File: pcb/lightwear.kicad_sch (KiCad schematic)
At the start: 21 parts, among them SW1 SW_SPST

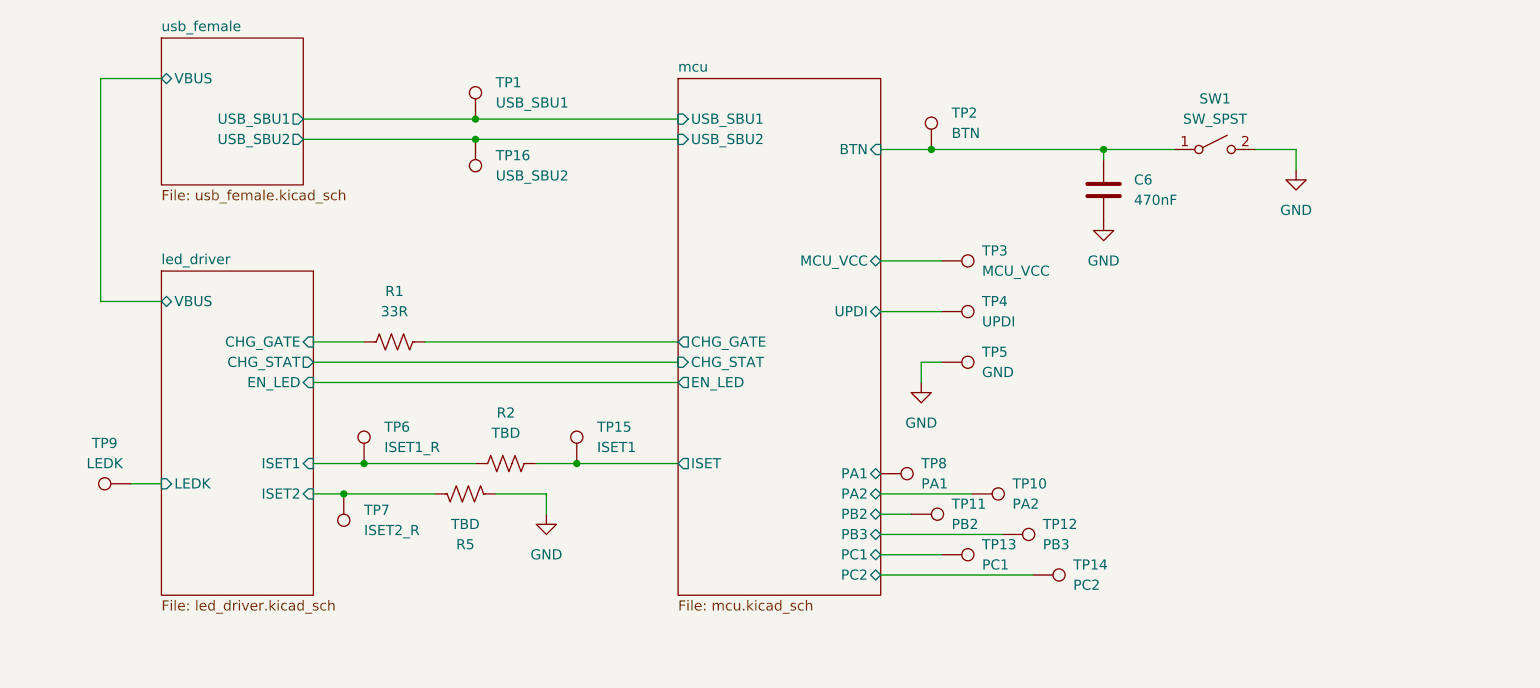
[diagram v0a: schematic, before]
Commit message: rev0 done
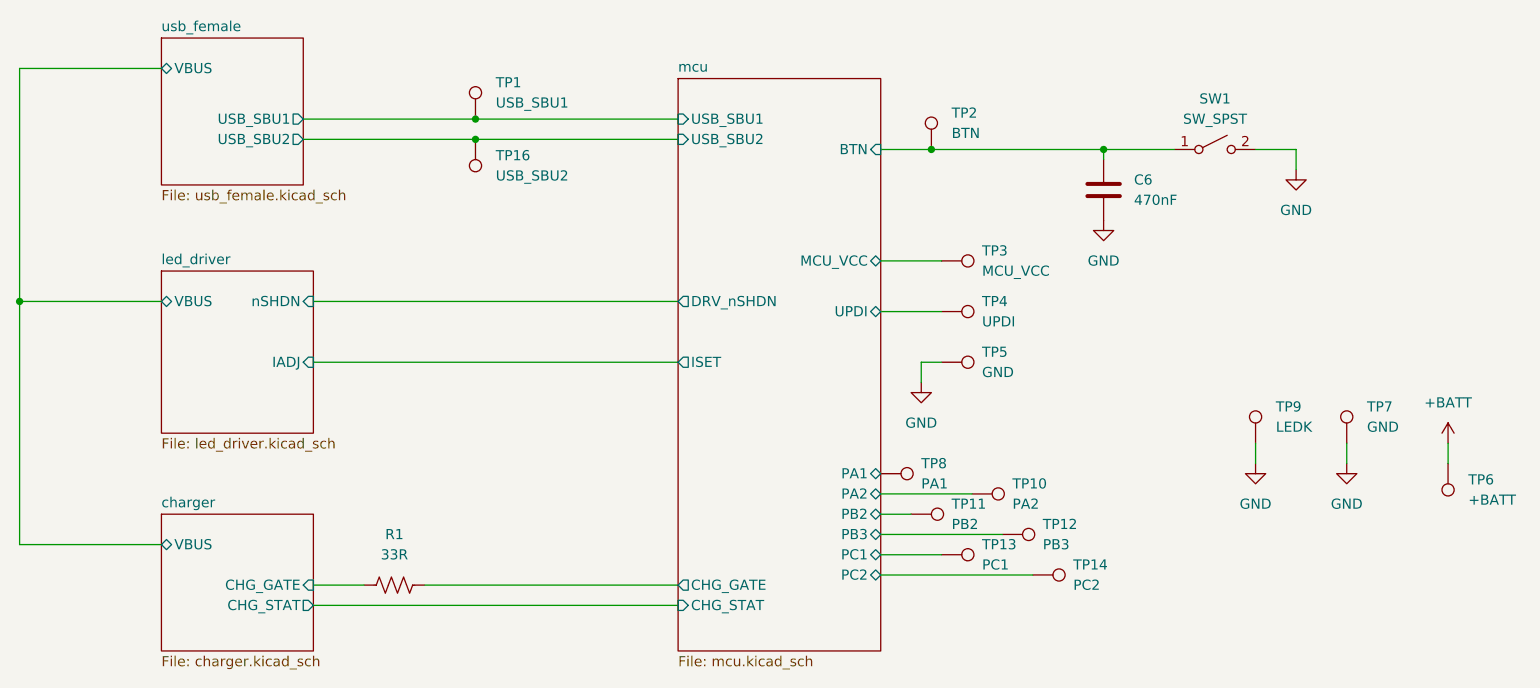
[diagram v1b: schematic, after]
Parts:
- removed R2, R5: TBD, Resistor_SMD:R_0402_1005Metric, symbol Device:R_US
- removed TP15: ISET1, symbol Connector:TestPoint
- SW1: footprint (none) -> footprints:SW4_PTS815 SJM 250 SMTR LFS_CNK
- TP1, TP10, TP11, TP12, TP13, TP14, TP16, TP2, TP8: footprint (none) -> TestPoint:TestPoint_Pad_D2.0mm
- TP3, TP4, TP5: footprint (none) -> TestPoint:TestPoint_Pad_D1.5mm
- TP6: value ISET1_R -> +BATT; footprint (none) -> TestPoint:TestPoint_Pad_1.5x1.5mm
- TP7: value ISET2_R -> GND; footprint (none) -> TestPoint:TestPoint_Pad_1.5x1.5mm
- TP9: footprint footprints:TestPoint_Pad_7.0x15.0mm -> footprints:TestPoint_Pad_6.0x12.0mm
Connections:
- net led_driver/ISET2 is gone; now on net GND: TP7.1
- net led_driver/LEDK is gone; now on net GND: TP9.1
- net led_driver/CHG_GATE renamed charger/CHG_GATE
- net led_driver/ISET1 renamed +BATT
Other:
- added sheet charger (charger.kicad_sch)
- sheet led_driver ports: added IADJ, nSHDN; removed CHG_GATE, CHG_STAT, EN_LED, ISET1, ISET2, LEDK
- sheet mcu ports: added DRV_nSHDN; removed EN_LED
- moved on the sheet: R1, TP9
